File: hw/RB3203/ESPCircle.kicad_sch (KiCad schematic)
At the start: 29 parts

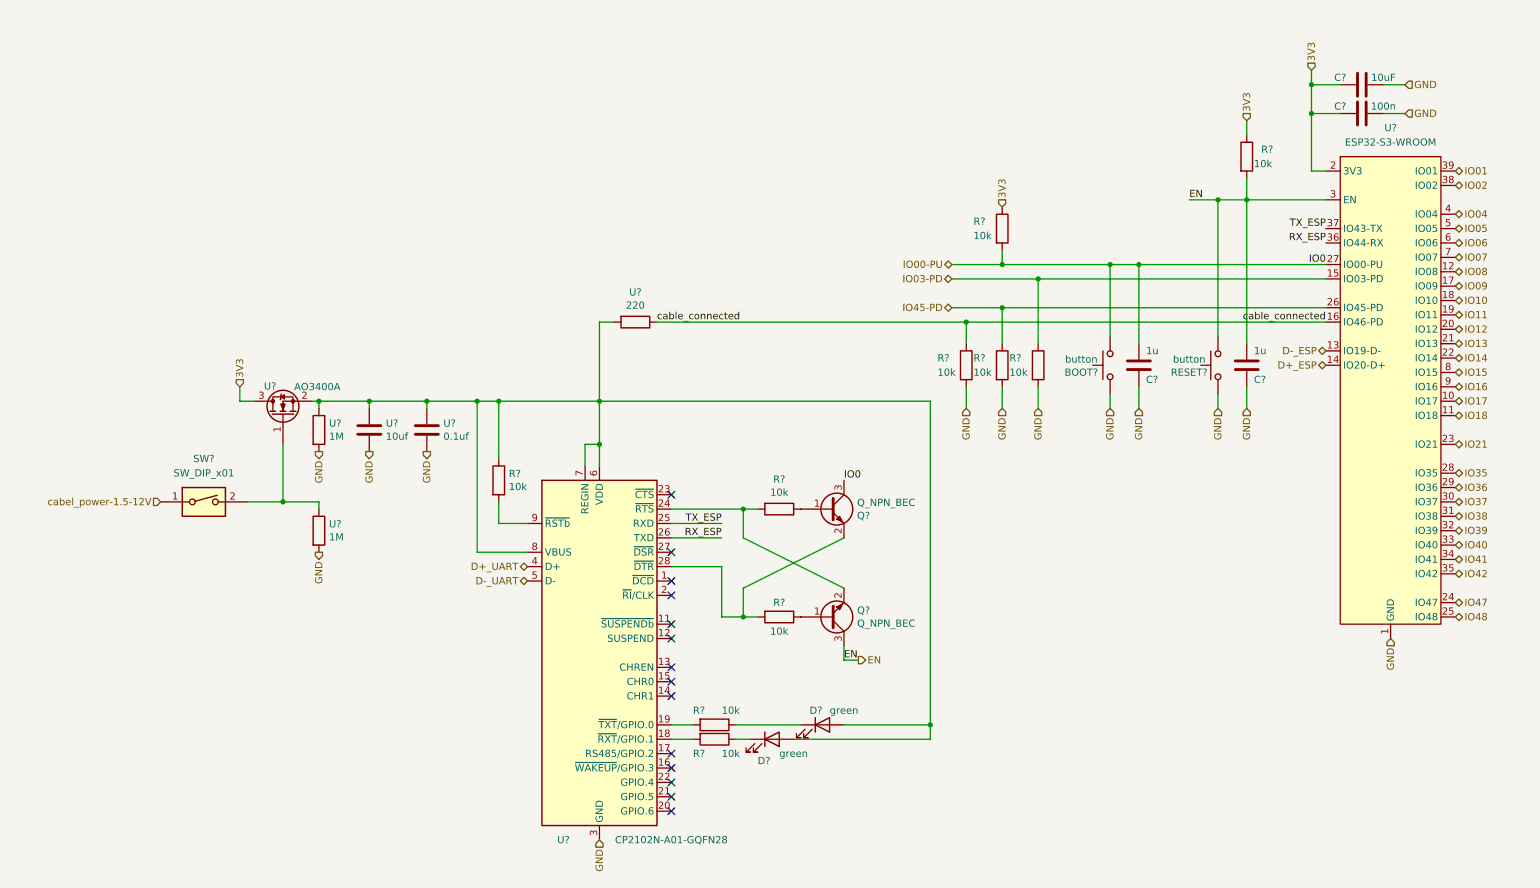
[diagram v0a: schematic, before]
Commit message: Wip
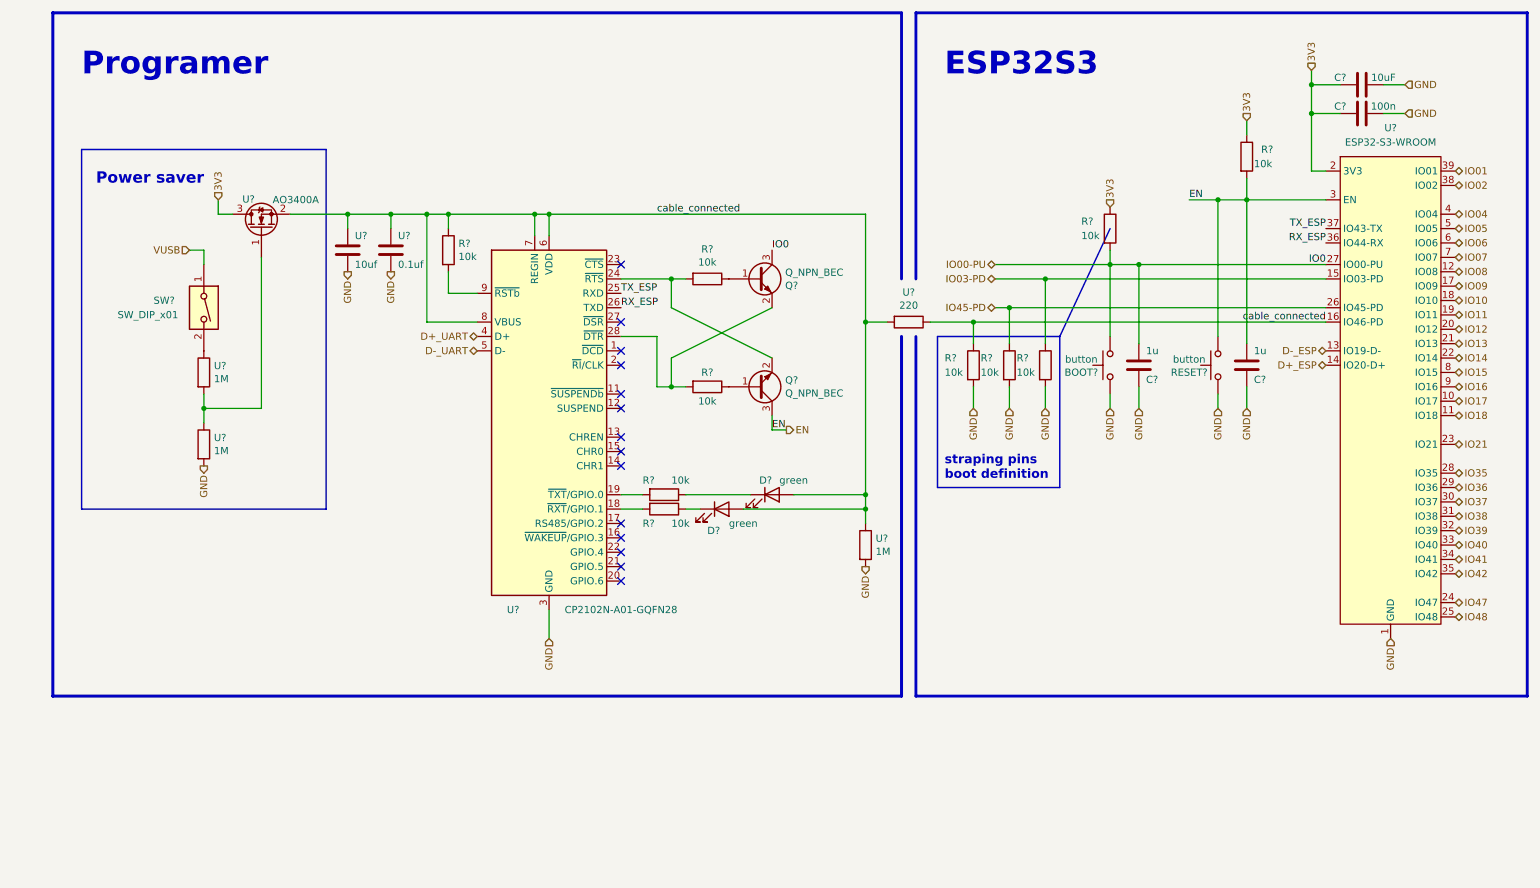
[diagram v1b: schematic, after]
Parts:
- added U?: 1M, Resistor_SMD:R_0402_1005Metric, symbol B.B-rescue:R-Device-B.B-rescue-B.B-rescue
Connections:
- net GND: now also U?.2; no longer U?.2
- net cable_connected: now also D?.2 (A), D?.2 (A), R?.1, U?.1, U?.1, U?.1, U?.2, U?.2 (S), U?.6 (VDD), U?.7 (REGIN), U?.8 (VBUS)
- net at SW?.2, U?.1: no longer U?.1 (G)
- net cabel_power-1.5-12V renamed VUSB
- new net: U?.1, U?.1 (G), U?.2
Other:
- note added: "ESP32S3"
- note added: "Power saver"
- note added: "Programer"
- note added: "straping pins boot definition"
- moved on the sheet: D?, Q?, R?, SW?, U?
